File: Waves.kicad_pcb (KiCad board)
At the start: 2 copper layers, 49.8 x 106.5 mm, 147 parts, among them J1 AudioJack2_SwitchT, J10 AudioJack2_SwitchT, J11 Conn_01x04_Male, J12 Conn_01x04_Male, J13 AudioJack2_SwitchT, J14 AudioJack2_SwitchT, J15 Conn_02x05_Odd_Even, J2 AudioJack2_SwitchT, J3 AudioJack2_SwitchT, J4 AudioJack2_SwitchT, J5 AudioJack2_SwitchT, J6 AudioJack2_SwitchT, J7 AudioJack2_SwitchT, J8 AudioJack2_SwitchT, J9 AudioJack2_SwitchT, Q1 BC847, Q2 BC847, Q3 BC847, Q4 BC847, Q5 BC847, SW1 SW_Push, SW2 Rotary_Encoder_Switch, SW3 SW_Push_LED, SW4 SW_Push_LED, SW5 SW_Push_LED, U1 STM32G431, U2 AT25xxx, U3 IPS240x240, U4 PCM5100, U5 TL072, U6 LM1117-3.3, U7 LM1117-3.3, U8 MCP6004, U9 MCP6004, Y1 8MHz

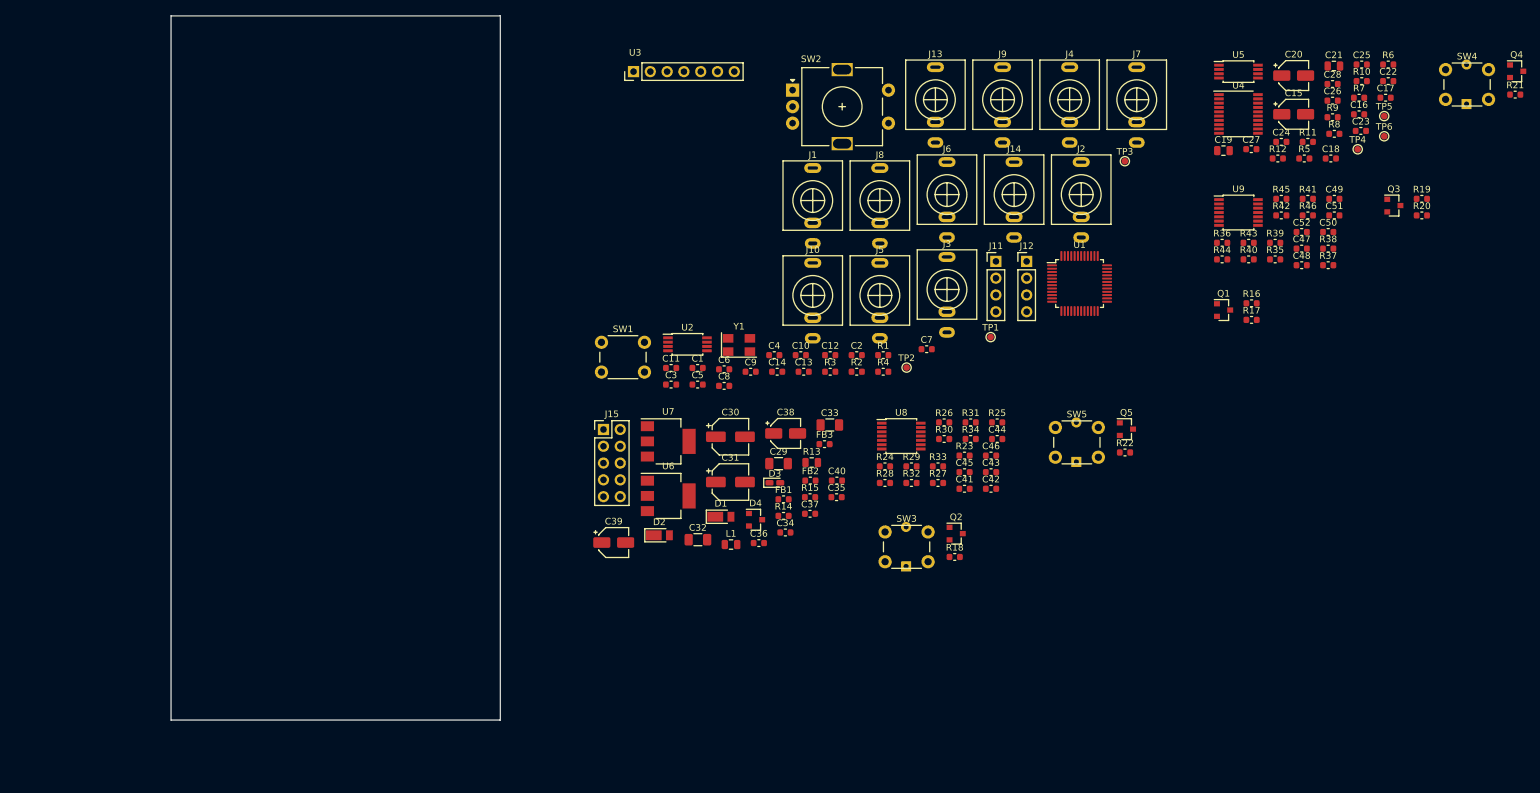
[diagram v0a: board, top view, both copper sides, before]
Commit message: Placed front-side components.
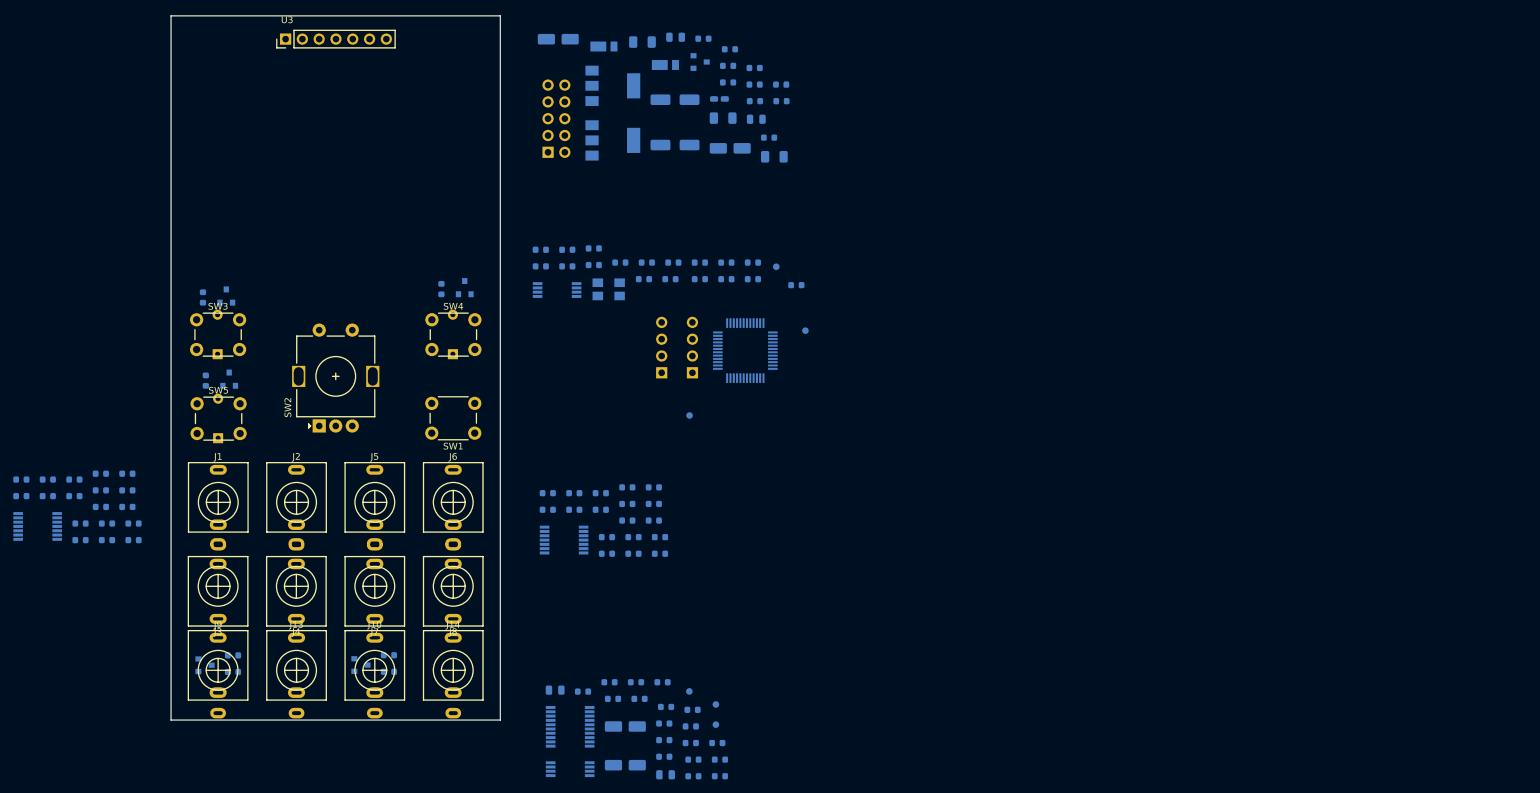
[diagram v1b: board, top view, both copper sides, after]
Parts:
- C1, C10, C11, C12, C13, C14, C15, C16, C17, C18, C19, C2, C20, C21, C22, C23, C24, C25, C26, C27, C28, C29, C3, C30, C31, C32, C33, C34, C35, C36, C37, C38, C39, C4, C40, C41, C42, C43, C44, C45, C46, C47, C48, C49, C5, C50, C51, C52, C6, C7, C8, C9, D1, D2, D3, D4, FB1, FB2, FB3, J11, J12, J15, L1, Q1, Q2, Q3, Q4, Q5, R1, R10, R11, R12, R13, R14, R15, R16, R17, R18, R19, R2, R20, R21, R22, R23, R24, R25, R26, R27, R28, R29, R3, R30, R31, R32, R33, R34, R35, R36, R37, R38, R39, R4, R40, R41, R42, R43, R44, R45, R46, R5, R6, R7, R8, R9, TP1, TP2, TP3, TP4, TP5, TP6, U1, U2, U4, U5, U6, U7, U8, U9, Y1: moved to B.Cu
- moved R19 193.5 mm to (111.3, 147.6)
- moved Q3 192.8 mm to (107.1, 146.6)
- moved R20 191.7 mm to (111.3, 145.1)
- moved R21 165.0 mm to (142.9, 89.7), turned to 90 degrees
- moved Q4 162.4 mm to (146.4, 89.4), turned to 90 degrees
- moved SW4 157.9 mm to (144.6, 96.6)
- moved C25 147.6 mm to (181.0, 163.3)
- moved R6 147.6 mm to (185.0, 163.3)
- moved C21 147.3 mm to (176.8, 163.1)
- moved J9 146.7 mm to (109.1, 147.3)
- moved U5 146.1 mm to (162.3, 162.3)
- moved C20 145.2 mm to (170.7, 161.7)
- moved C22 144.0 mm to (185.0, 160.8)
- moved R10 144.0 mm to (181.0, 160.8)
- moved C28 143.4 mm to (176.6, 160.4)
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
